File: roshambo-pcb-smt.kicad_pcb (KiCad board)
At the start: 2 copper layers, 49 parts, among them J1 Conn_01x06_Socket, J2 Conn_01x03_Pin, J3 Conn_01x03_Pin, Q1 2N7002, Q2 2N7002, Q3 2N7002, Q4 2N7002, Q5 2N7002, Q6 2N7002, Q7 2N7002, Q8 2N7002, Q9 2N7002, U1 Pico

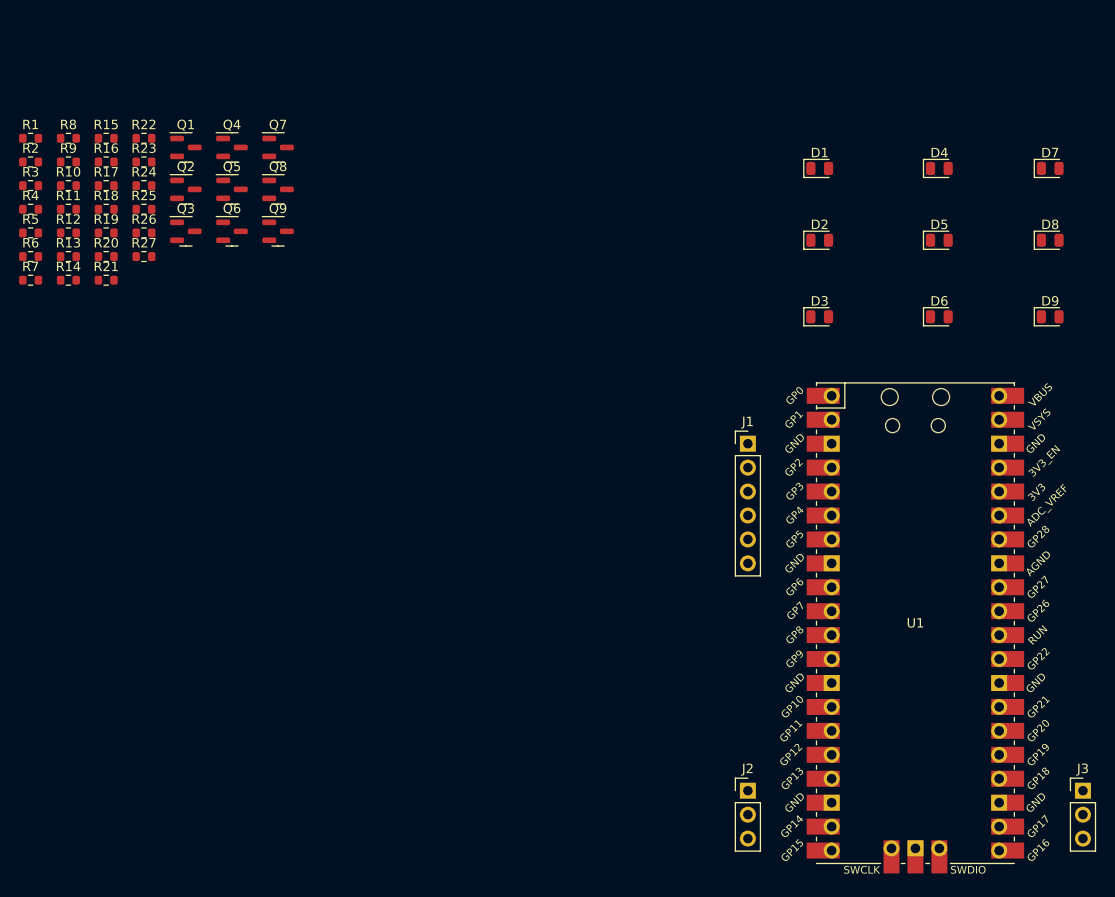
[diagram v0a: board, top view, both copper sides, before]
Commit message: More progress on the layout
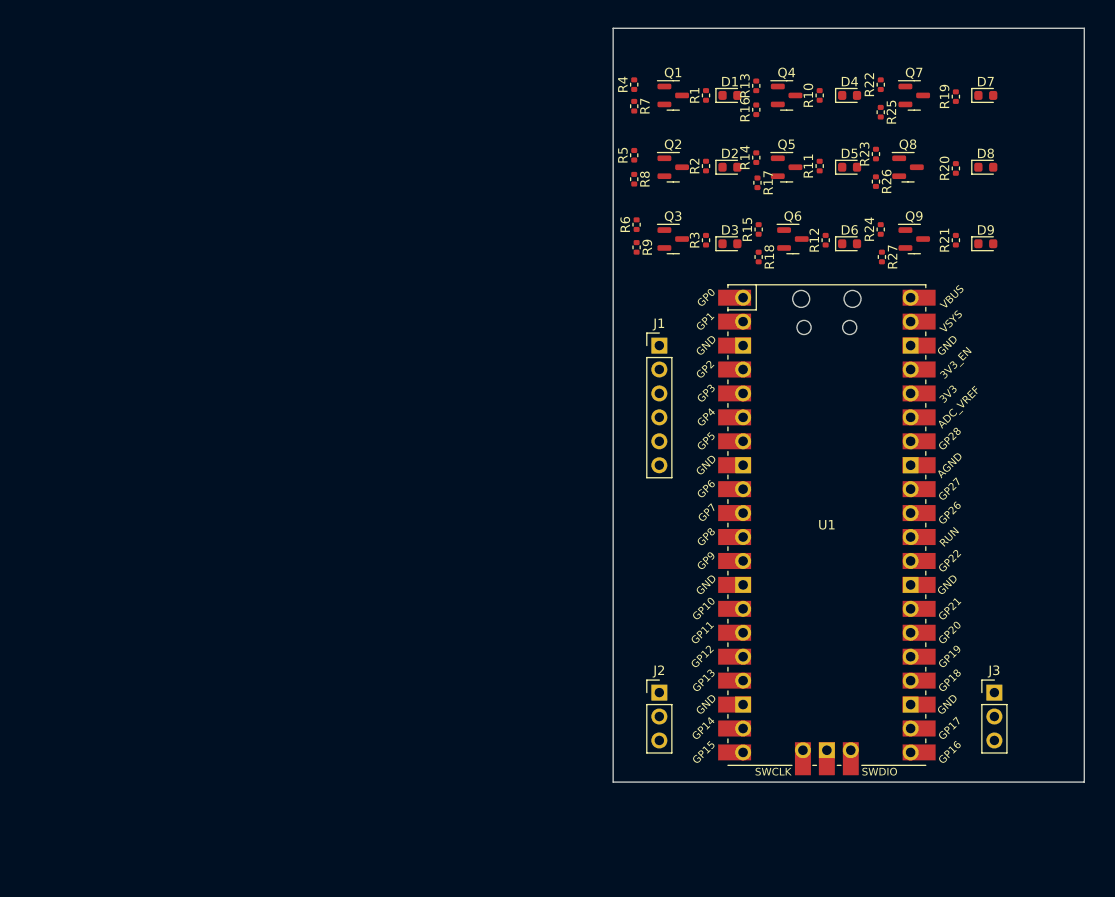
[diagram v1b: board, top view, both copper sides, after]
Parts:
- D1, D2, D3, D4, D5, D6, D7, D8, D9: footprint LED_SMD:LED_0805_2012Metric -> LED_SMD:LED_0603_1608Metric
- R1, R10, R11, R12, R13, R14, R15, R16, R17, R18, R19, R2, R20, R21, R22, R23, R24, R25, R26, R27, R3, R4, R5, R6, R7, R8, R9: footprint Resistor_SMD:R_0603_1608Metric -> Resistor_SMD:R_0402_1005Metric
- moved R19 91.3 mm to (133.8, 35.6), turned to 90 degrees
- moved R20 90.7 mm to (133.8, 43.2), turned to 90 degrees
- moved R21 90.3 mm to (133.8, 50.8), turned to 90 degrees
- moved R12 80.4 mm to (120.0, 50.8), turned to 90 degrees
- moved R10 80.3 mm to (119.4, 35.4), turned to 90 degrees
- moved R11 79.9 mm to (119.4, 42.9), turned to 90 degrees
- moved R25 78.9 mm to (125.9, 37.2), turned to -90 degrees
- moved R22 78.4 mm to (125.9, 34.3), turned to 90 degrees
- moved R24 78.3 mm to (125.9, 49.7), turned to 90 degrees
- moved R27 78.3 mm to (126.0, 52.6), turned to -90 degrees
- moved R26 77.9 mm to (125.3, 44.6), turned to -90 degrees
- moved R23 77.7 mm to (125.4, 41.7), turned to 90 degrees
- moved R13 75.2 mm to (112.6, 34.4), turned to 90 degrees
- moved R14 74.2 mm to (112.6, 42.0), turned to 90 degrees
- moved R3 71.9 mm to (107.3, 50.8), turned to 90 degrees
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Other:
- board outline added: 50 x 80 mm

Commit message: Released to Production
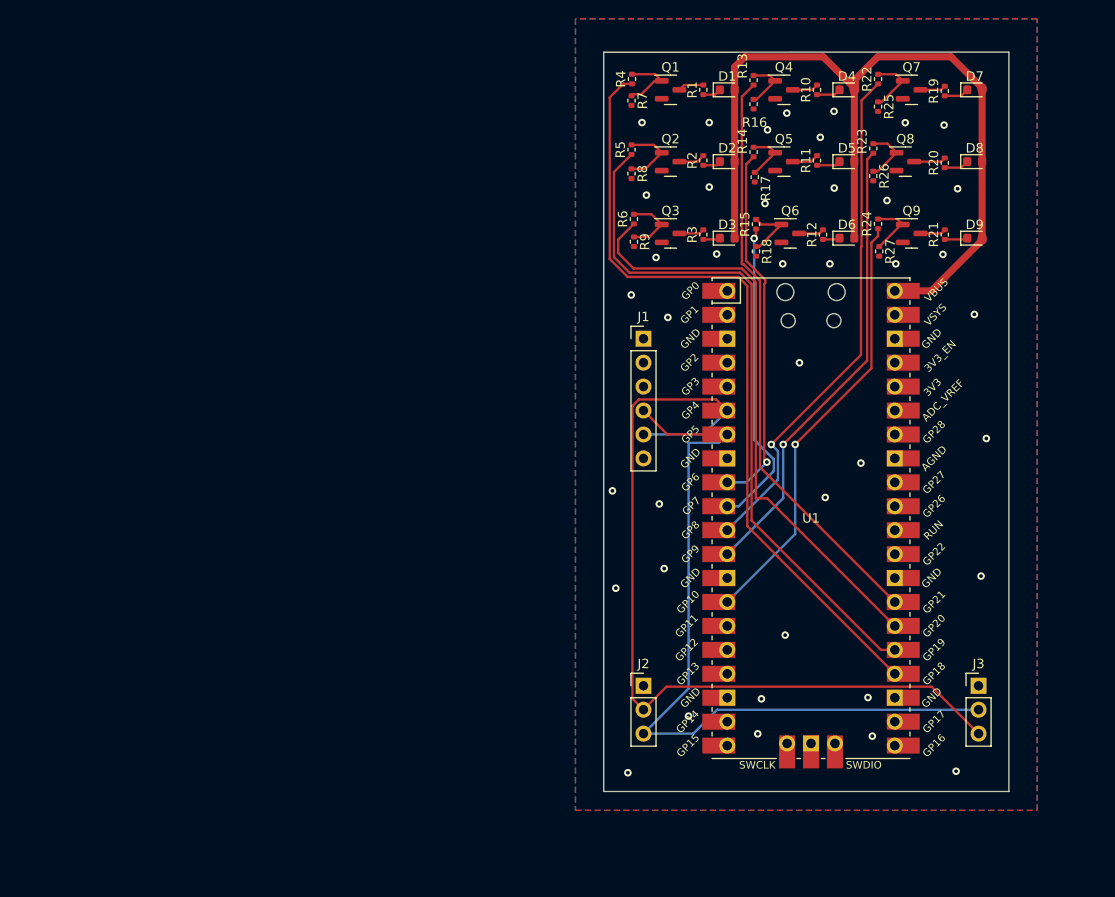
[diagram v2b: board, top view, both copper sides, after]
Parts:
- D1, D4, D7: value LED -> RED
- D2, D5, D9: value LED -> GREEN
- D3, D6: value LED -> BLUE
- D8: value LED -> YELLOW
- R1, R10, R19, R20: value 47 -> 150
- R11, R2, R21: value 47 -> 40
- R12, R3: value 47 -> 88
- moved U1 1.83 mm to (118.5, 80.3)
- moved J2 1.83 mm to (100.7, 98.1)
- moved J3 1.83 mm to (136.2, 98.1)
- moved J1 1.83 mm to (100.7, 61.3)
- moved R19 1.32 mm to (132.7, 35.0)
- moved R20 1.32 mm to (132.7, 42.6)
- moved R21 1.32 mm to (132.7, 50.2)
- moved D7 1.32 mm to (135.8, 34.8)
- moved D8 1.32 mm to (135.8, 42.5)
- moved D9 1.32 mm to (135.8, 50.6)
- moved R16 0.66 mm to (112.4, 36.4), turned to -90 degrees
- moved R17 0.66 mm to (112.5, 44.1)
- moved R18 0.66 mm to (112.6, 52.0)
- moved R23 0.66 mm to (125.1, 41.1)
- moved R6 0.66 mm to (99.7, 48.5)
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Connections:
- Q9 pad 1: GND -> Net-(Q9-G)
- R24 pad 2: GND -> Net-(Q9-G)
- R27 pad 1: GND -> Net-(Q9-G)
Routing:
- net +5V: track 0.00 -> 93.2 mm
- net /TX1: track 0.00 -> 92.1 mm
- net /RX1: track 0.00 -> 83.9 mm
- net /PWM1A: track 0.00 -> 83.5 mm
- net /PWM1B: track 0.00 -> 73.4 mm
- net /PWM2A: track 0.00 -> 62.9 mm
- net /PWM2B: track 0.00 -> 62.2 mm
- net /PWM4A: track 0.00 -> 54.6 mm, vias 0 -> 1
- net /PWM4B: track 0.00 -> 49.0 mm, vias 0 -> 1
- net /PWM5A: track 0.00 -> 46.3 mm, vias 0 -> 1
- net /PWM3A: track 0.00 -> 38.8 mm, vias 0 -> 1
- net /PWM3B: track 0.00 -> 33.1 mm, vias 0 -> 1
- net Net-(Q2-G): track 0.00 -> 7.46 mm
- net Net-(Q1-G): track 0.00 -> 7.38 mm
- net Net-(Q3-G): track 0.00 -> 6.90 mm
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- added copper zone on B.Cu, net GND
- added copper zone on F.Cu, net GND
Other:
- board size 50 x 80 mm -> 43 x 78.5 mm
